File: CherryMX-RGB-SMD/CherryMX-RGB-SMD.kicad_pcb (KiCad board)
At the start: 2 copper layers, 17.8 x 17.8 mm, 5 parts, among them P1 CONN_01X07, SW1 SW_PUSH, U1 11AA010T

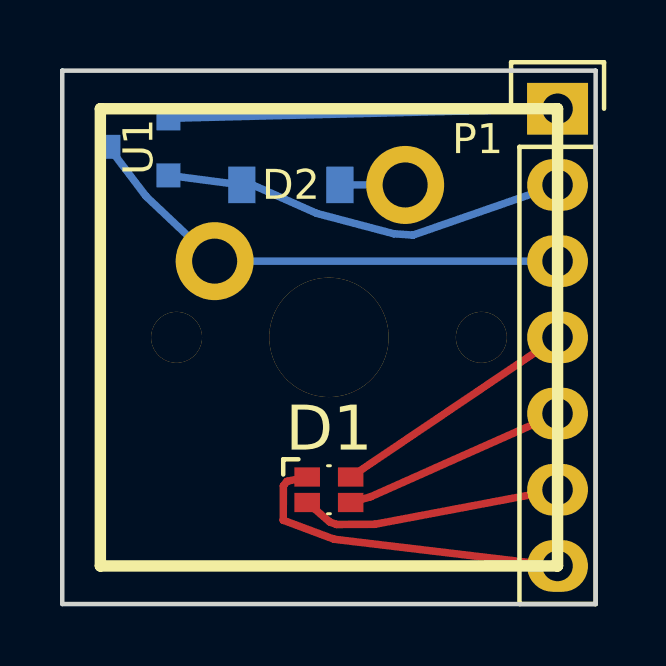
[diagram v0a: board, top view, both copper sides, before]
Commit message: Minor cleanups
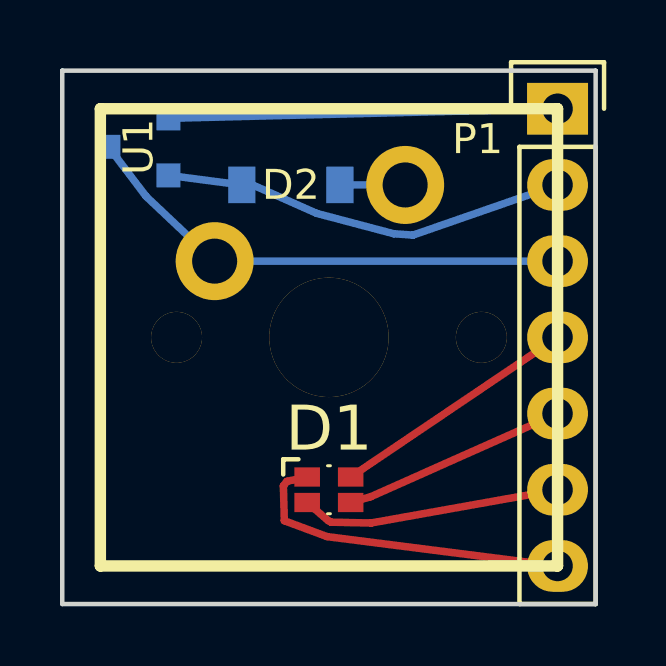
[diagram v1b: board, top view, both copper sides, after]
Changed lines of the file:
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@@
     (links 10)
     (no_connects 0)
-    (area -8.965001 -8.965001 8.965001 8.965001)
+    (area -8.965001 -11.845 12.728334 10.6267)
     (thickness 1.6)
     (drawings 4)
@@
   (segment (start 0.725 5.505) (end 1.390995 5.313155) (width 0.25) (layer F.Cu) (net 5) (status 10))
   (segment (start 1.390995 5.313155) (end 7.62 2.54) (width 0.25) (layer F.Cu) (net 5) (status 20))
-  (segment (start -0.725 5.505) (end 0.025679 6.153521) (width 0.25) (layer F.Cu) (net 6) (status 10))
-  (segment (start 1.525667 6.231821) (end 7.62 5.08) (width 0.25) (layer F.Cu) (net 6) (status 20))
-  (segment (start 0.254072 6.237933) (end 1.525667 6.231821) (width 0.25) (layer F.Cu) (net 6))
-  (segment (start 0.025679 6.153521) (end 0.254072 6.237933) (width 0.25) (layer F.Cu) (net 6))
+  (segment (start -0.725 5.505) (end -0.026732 6.108241) (width 0.25) (layer F.Cu) (net 6) (status 400010))
+  (segment (start 1.404462 6.188633) (end 7.62 5.08) (width 0.25) (layer F.Cu) (net 6) (status 800020))
+  (segment (start 0.072106 6.161151) (end 1.404462 6.188633) (width 0.25) (layer F.Cu) (net 6))
+  (segment (start -0.026732 6.108241) (end 0.072106 6.161151) (width 0.25) (layer F.Cu) (net 6))
   (segment (start 0.725 4.655) (end 7.62 0) (width 0.25) (layer F.Cu) (net 7) (status 30))
   (segment (start -0.725 4.655) (end -1.402562 4.80001) (width 0.25) (layer F.Cu) (net 8) (status 10))
-  (segment (start 0.17171 6.729428) (end 7.62 7.62) (width 0.25) (layer F.Cu) (net 8) (status 20))
-  (segment (start -1.524 6.096) (end 0.17171 6.729428) (width 0.25) (layer F.Cu) (net 8))
-  (segment (start -1.519 4.952803) (end -1.524 6.096) (width 0.25) (layer F.Cu) (net 8))
+  (segment (start -0.063458 6.641988) (end 7.62 7.62) (width 0.25) (layer F.Cu) (net 8) (status 800020))
+  (segment (start -1.487337 6.112566) (end -0.063458 6.641988) (width 0.25) (layer F.Cu) (net 8))
+  (segment (start -1.519 4.952803) (end -1.487337 6.112566) (width 0.25) (layer F.Cu) (net 8))
   (segment (start -1.402562 4.80001) (end -1.519 4.952803) (width 0.25) (layer F.Cu) (net 8))
 )
